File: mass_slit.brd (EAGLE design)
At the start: 37.8 x 39.4 mm, 31 parts, among them IC1 PIC18F1220P

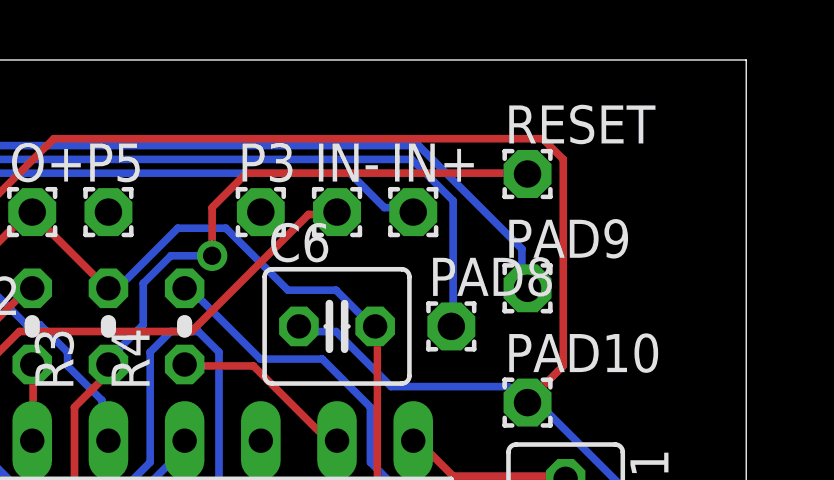
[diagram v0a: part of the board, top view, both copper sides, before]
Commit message: up
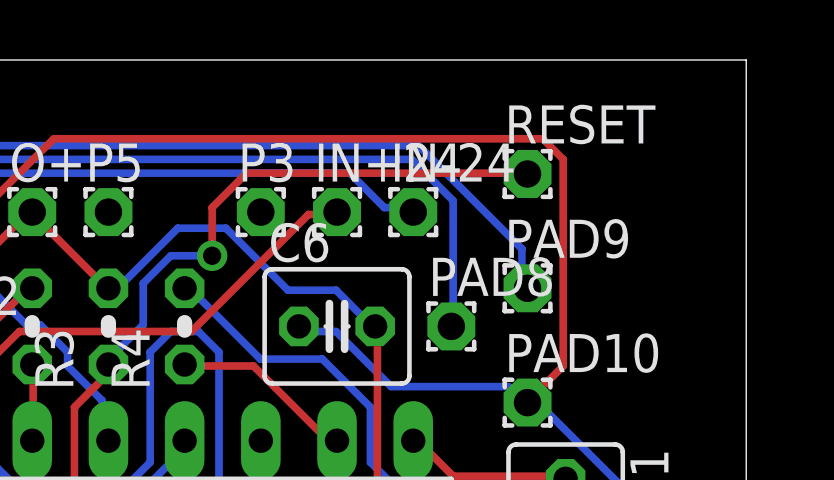
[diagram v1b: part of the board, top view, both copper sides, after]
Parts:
- C1, C4, C6: value (none) -> 10uf
- C3, C5: value (none) -> 0.1
- R1: value (none) -> 2000
- R2, R4, R5: value (none) -> 220
- R3: value (none) -> 10000
- renumbered IN+ to IN-24, IN- to IN+24
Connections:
- net N$5 renamed -24
- net N$6 renamed +24
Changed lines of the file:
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@@
 <?xml version="1.0" encoding="utf-8"?>
 <!DOCTYPE eagle SYSTEM "eagle.dtd">
-<eagle version="9.2.2">
+<eagle version="9.4.1">
 <drawing>
 <settings>
@@
 <attribute name="VALUE" x="21.59" y="32.35" size="0.0254" layer="27"/>
 </element>
-<element name="IN-" library="wirepad" package="1,6/0,9" value="" x="24.13" y="31.75" smashed="yes">
+<element name="IN+24" library="wirepad" package="1,6/0,9" value="" x="24.13" y="31.75" smashed="yes">
 <attribute name="NAME" x="23.368" y="32.766" size="1.27" layer="25" ratio="10"/>
 <attribute name="VALUE" x="24.13" y="32.35" size="0.0254" layer="27"/>
 </element>
-<element name="IN+" library="wirepad" package="1,6/0,9" value="" x="26.67" y="31.75" smashed="yes">
+<element name="IN-24" library="wirepad" package="1,6/0,9" value="" x="26.67" y="31.75" smashed="yes">
 <attribute name="NAME" x="25.908" y="32.766" size="1.27" layer="25" ratio="10"/>
 <attribute name="VALUE" x="26.67" y="32.35" size="0.0254" layer="27"/>
 </element>
-<element name="C1" library="resistor" package="C025-040X050" value="" x="31.75" y="21.59" smashed="yes" rot="R270">
+<element name="C1" library="resistor" package="C025-040X050" value="10uf" x="31.75" y="21.59" smashed="yes" rot="R270">
 <attribute name="NAME" x="33.909" y="23.876" size="1.27" layer="25" ratio="10" rot="R270"/>
 <attribute name="VALUE" x="28.321" y="23.876" size="1.27" layer="27" ratio="10" rot="R270"/>
 </element>
-<element name="C3" library="capacitor-wima" package="C5B2.5" value="" x="30.48" y="10.16" smashed="yes">
+<element name="C3" library="capacitor-wima" package="C5B2.5" value="0.1" x="30.48" y="10.16" smashed="yes">
 <attribute name="NAME" x="28.448" y="11.684" size="1.27" layer="25" ratio="10"/>
 <attribute name="VALUE" x="28.448" y="7.366" size="1.27" layer="27" ratio="10"/>
 </element>
-<element name="C4" library="resistor" package="C025-040X050" value="" x="7.62" y="12.7" smashed="yes">
+<element name="C4" library="resistor" package="C025-040X050" value="10uf" x="7.62" y="12.7" smashed="yes">
 <attribute name="NAME" x="5.334" y="14.859" size="1.27" layer="25" ratio="10"/>
 <attribute name="VALUE" x="5.334" y="9.271" size="1.27" layer="27" ratio="10"/>
 </element>
-<element name="C5" library="capacitor-wima" package="C5B2.5" value="" x="19.05" y="12.7" smashed="yes">
+<element name="C5" library="capacitor-wima" package="C5B2.5" value="0.1" x="19.05" y="12.7" smashed="yes">
 <attribute name="NAME" x="17.018" y="14.224" size="1.27" layer="25" ratio="10"/>
 <attribute name="VALUE" x="17.018" y="9.906" size="1.27" layer="27" ratio="10"/>
 </element>
-<element name="C6" library="resistor" package="C025-040X050" value="" x="24.13" y="27.94" smashed="yes">
+<element name="C6" library="resistor" package="C025-040X050" value="10uf" x="24.13" y="27.94" smashed="yes">
 <attribute name="NAME" x="21.844" y="30.099" size="1.27" layer="25" ratio="10"/>
 <attribute name="VALUE" x="21.844" y="24.511" size="1.27" layer="27" ratio="10"/>
@@
 <attribute name="VALUE" x="5.1638" y="11.1407" size="1.27" layer="27"/>
 </element>
-<element name="R1" library="resistor" package="RTRIM3339P" value="" x="30.48" y="3.81" smashed="yes" rot="R180">
+<element name="R1" library="resistor" package="RTRIM3339P" value="2000" x="30.48" y="3.81" smashed="yes" rot="R180">
 <attribute name="NAME" x="32.995" y="-0.395" size="1.27" layer="25" rot="R180"/>
 <attribute name="VALUE" x="32.995" y="9.415" size="1.27" layer="27" rot="R180"/>
 </element>
-<element name="R2" library="resistor" package="0204V" value="" x="12.7" y="12.7" smashed="yes">
+<element name="R2" library="resistor" package="0204V" value="220" x="12.7" y="12.7" smashed="yes">
 <attribute name="NAME" x="10.5664" y="13.8684" size="1.27" layer="25" ratio="10"/>
 <attribute name="VALUE" x="10.5664" y="10.3886" size="1.27" layer="27" ratio="10"/>
 </element>
-<element name="R3" library="resistor" package="0204V" value="" x="16.51" y="27.94" smashed="yes" rot="R90">
+<element name="R3" library="resistor" package="0204V" value="10000" x="16.51" y="27.94" smashed="yes" rot="R90">
 <attribute name="NAME" x="15.3416" y="25.8064" size="1.27" layer="25" ratio="10" rot="R90"/>
 <attribute name="VALUE" x="18.8214" y="25.8064" size="1.27" layer="27" ratio="10" rot="R90"/>
 </element>
-<element name="R4" library="resistor" package="0204V" value="" x="19.05" y="27.94" smashed="yes" rot="R90">
+<element name="R4" library="resistor" package="0204V" value="220" x="19.05" y="27.94" smashed="yes" rot="R90">
 <attribute name="NAME" x="17.8816" y="25.8064" size="1.27" layer="25" ratio="10" rot="R90"/>
 <attribute name="VALUE" x="21.3614" y="25.8064" size="1.27" layer="27" ratio="10" rot="R90"/>
@@
 <attribute name="VALUE" x="30.48" y="33.62" size="0.0254" layer="27"/>
 </element>
-<element name="R5" library="resistor" package="0204V" value="" x="13.97" y="27.94" smashed="yes" rot="R90">
+<element name="R5" library="resistor" package="0204V" value="220" x="13.97" y="27.94" smashed="yes" rot="R90">
 <attribute name="NAME" x="12.8016" y="25.8064" size="1.27" layer="25" ratio="10" rot="R90"/>
 <attribute name="VALUE" x="16.2814" y="25.8064" size="1.27" layer="27" ratio="10" rot="R90"/>
@@
 <wire x1="31.9005" y1="20.196" x2="31.75" y2="20.32" width="0.254" layer="1"/>
 </signal>
-<signal name="N$5">
-<contactref element="IN+" pad="1"/>
+<signal name="-24">
+<contactref element="IN-24" pad="1"/>
 <contactref element="C4" pad="1"/>
 <contactref element="J1" pad="7"/>
@@
 <wire x1="6.426" y1="12.852" x2="6.35" y2="12.7" width="0.254" layer="16"/>
 </signal>
-<signal name="N$6">
-<contactref element="IN-" pad="1"/>
+<signal name="+24">
+<contactref element="IN+24" pad="1"/>
 <contactref element="C4" pad="2"/>
 <contactref element="J1" pad="8"/>
